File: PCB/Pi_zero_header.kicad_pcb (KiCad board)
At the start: 2 copper layers, 30 x 65 mm, 103 parts, among them J1 Raspberry_Pi_2_3, J2 USB_C_Receptacle_USB2.0, J3 Screw_Terminal_01x02, J4 Screw_Terminal_01x02, J5 Conn_02x04_Top_Bottom, J6 Conn_01x07, J7 Conn_01x02, J8 Conn_02x03_Top_Bottom, J9 Conn_01x02, SW1 SW_Push, SW2 SW_Push, U1 RP2040, U2 W25Q128JVS, U3 TB6612FNG, U4 TPS630701RNMR, U5 TPS630701RNMR, U6 PQ25792RQMR, Y2 12M

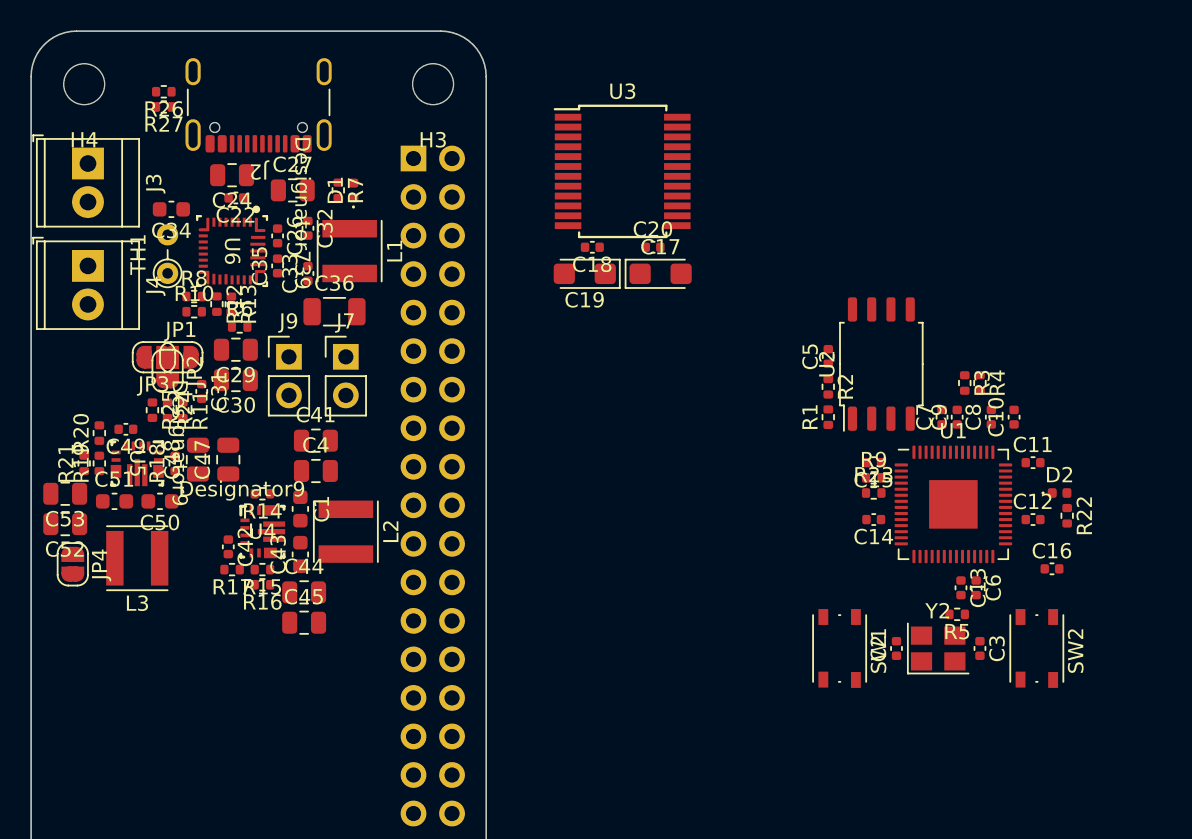
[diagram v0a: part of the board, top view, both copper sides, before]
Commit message: Getting somewhere...
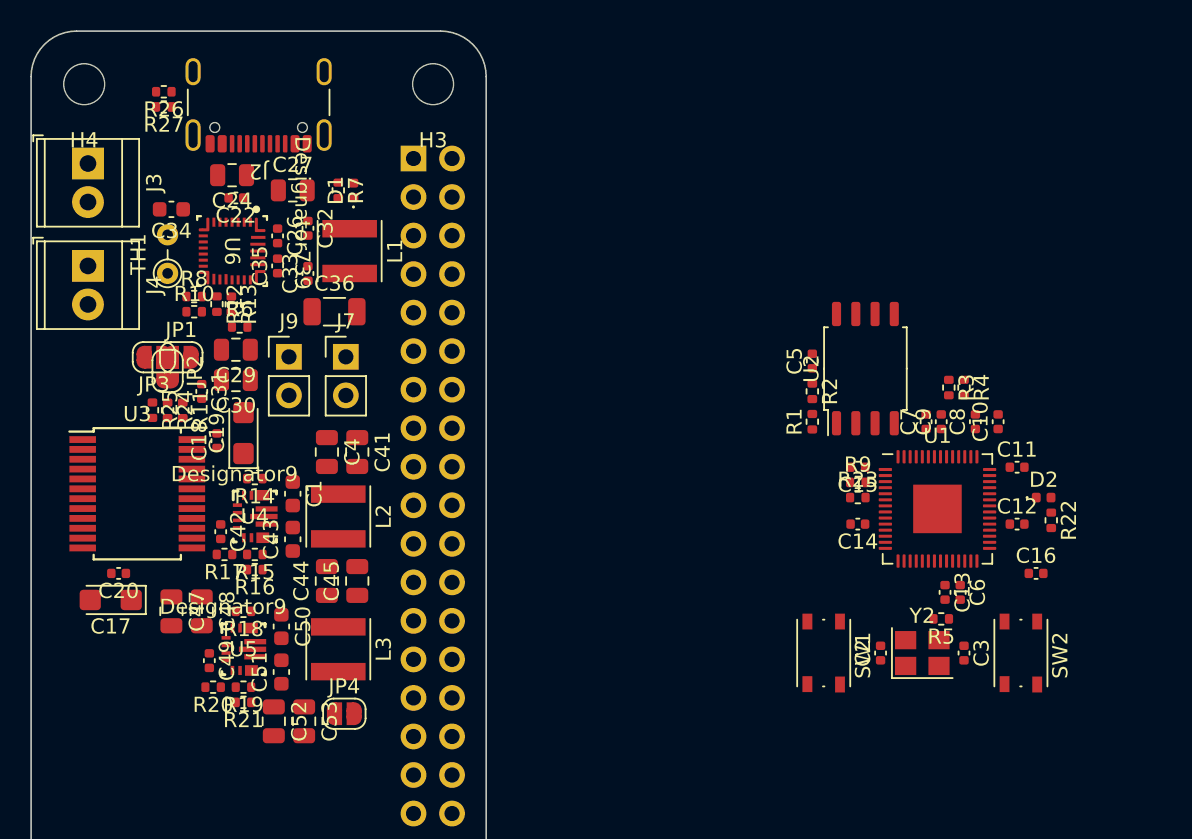
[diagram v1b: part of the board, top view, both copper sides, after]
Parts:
- moved C17 42.1 mm to (45.2, 90.0), turned to 180 degrees
- moved C20 41.3 mm to (45.8, 88.2), turned to 180 degrees
- moved U3 38.4 mm to (47.0, 83.0)
- moved C18 27.8 mm to (52.2, 79.5), turned to 90 degrees
- moved C19 24.8 mm to (54.0, 79.0), turned to 90 degrees
- moved C53 21.8 mm to (58.0, 98.0), turned to -90 degrees
- moved JP4 20.4 mm to (60.6, 97.5), turned to 0 degrees
- moved R21 18.9 mm to (54.0, 96.8), turned to 180 degrees
- moved C52 18.9 mm to (56.0, 98.0), turned to -90 degrees
- moved R20 18.4 mm to (52.0, 95.8), turned to 180 degrees
- moved R19 17.5 mm to (54.0, 95.8), turned to 180 degrees
- moved C49 16.2 mm to (51.8, 94.0), turned to -90 degrees
- moved C51 15.7 mm to (56.5, 94.8), turned to 90 degrees
- moved L3 14.5 mm to (60.2, 93.2), turned to -90 degrees
- moved U5 14.1 mm to (54.0, 93.2), turned to 0 degrees
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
